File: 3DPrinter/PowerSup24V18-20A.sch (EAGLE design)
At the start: 77 parts, among them IC1 POWER-TNY264PN, T1 TRANS-1/1EFD25-10, T2 _TRANSFORMERS_GDT_20X6.5, T3 TRANS-1/1ETD39, U1 SG3525AN, X1 CON-7.62-02P, X2 CON-7.62-02P

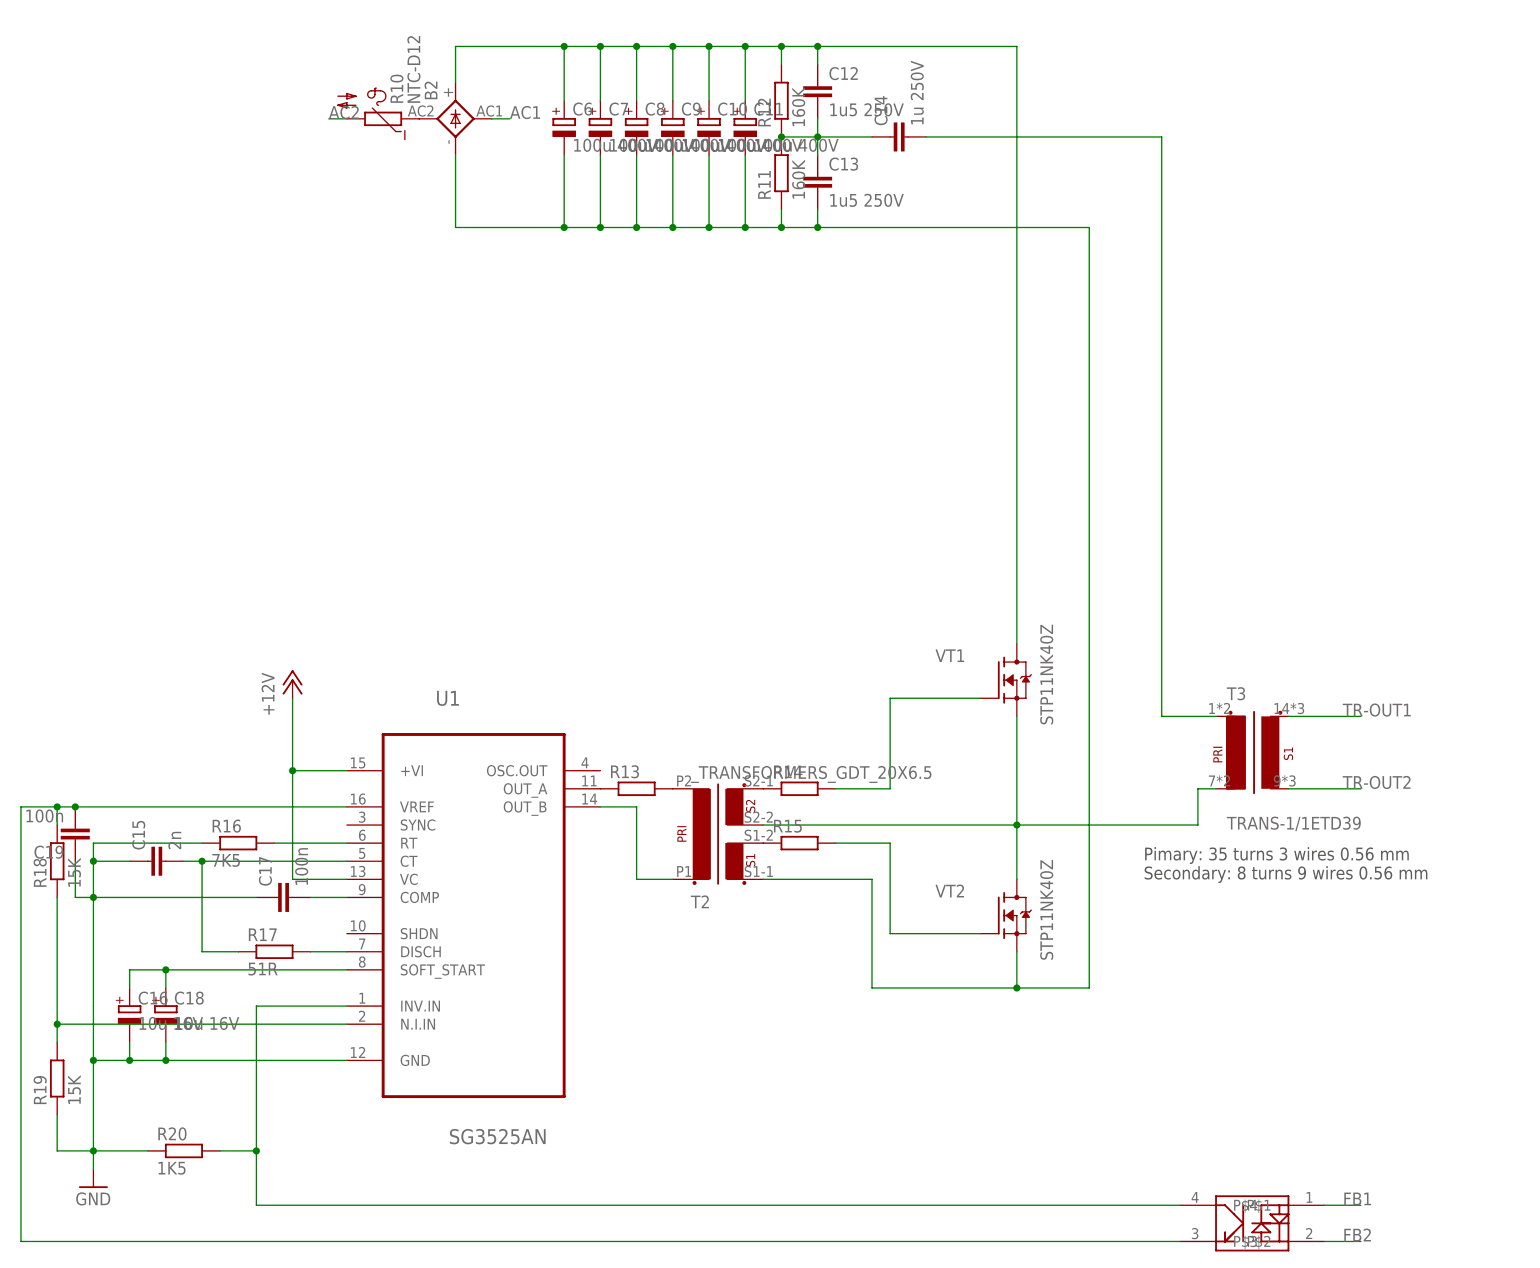
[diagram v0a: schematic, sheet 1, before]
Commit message: как всегда
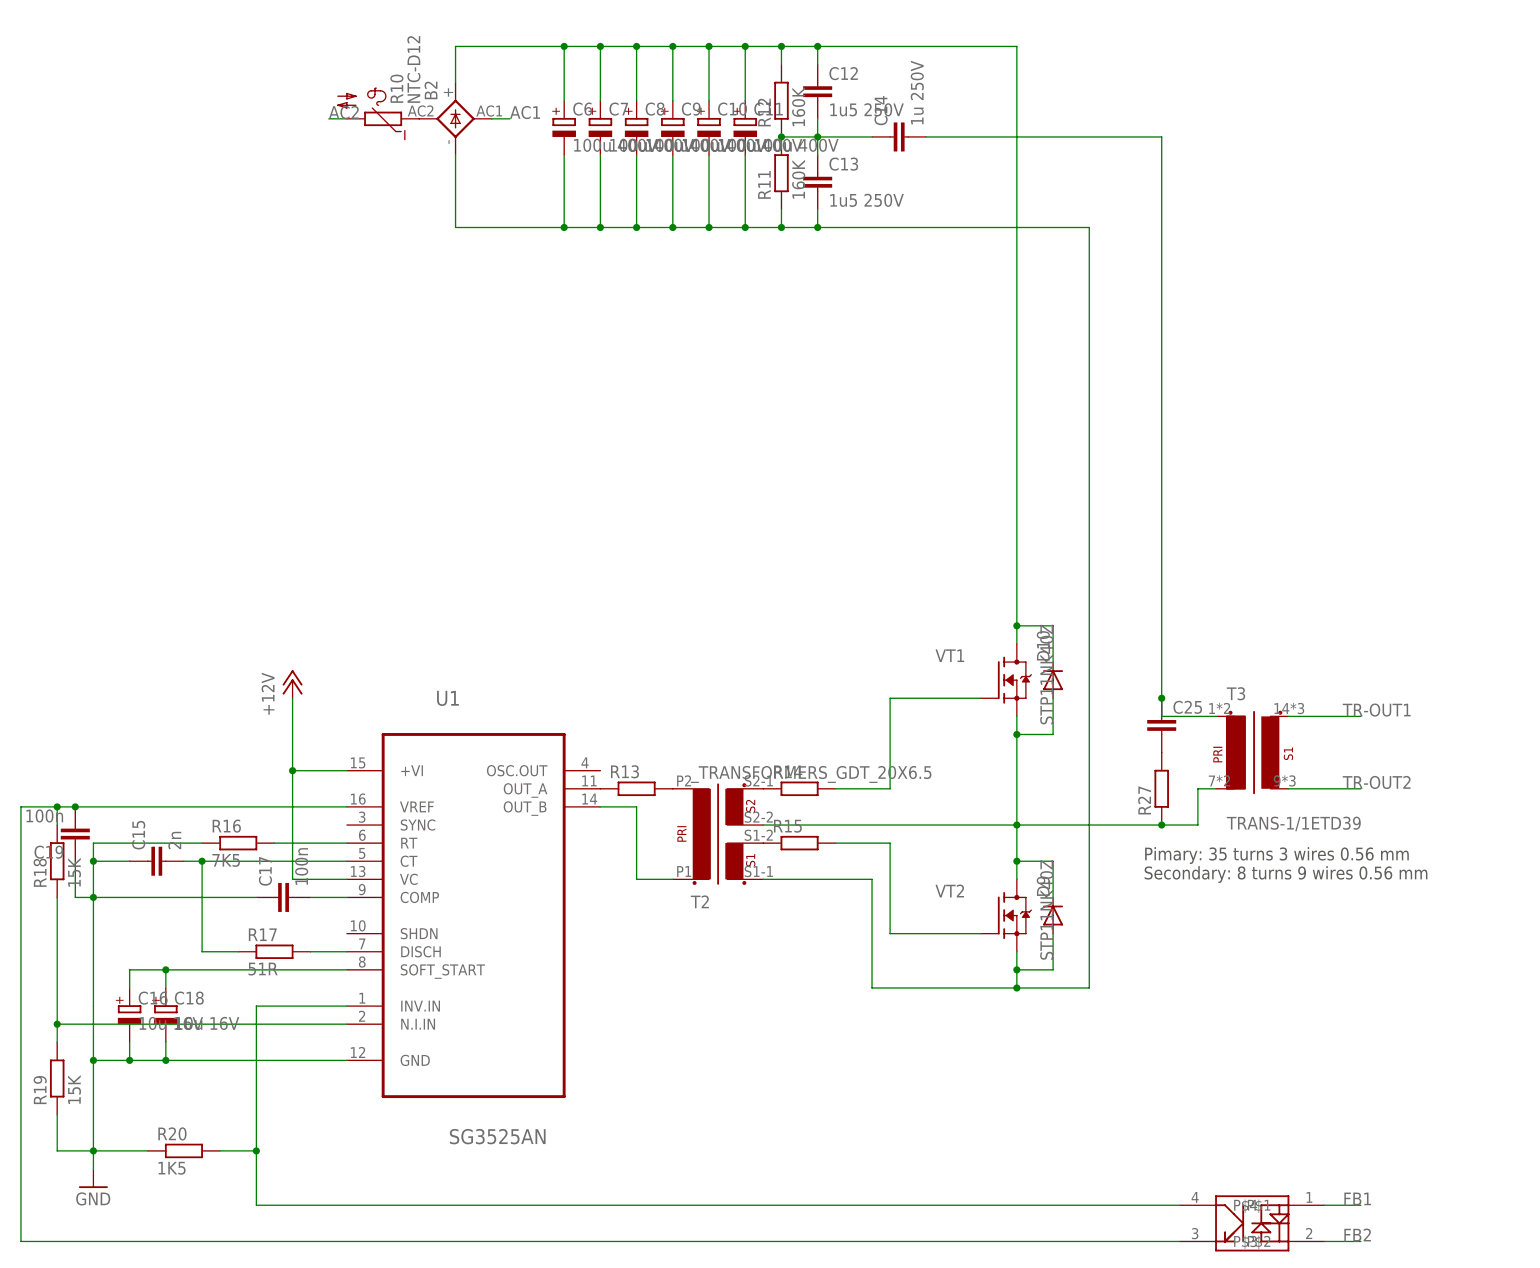
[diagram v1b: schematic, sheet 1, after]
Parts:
- added C25: (no value), Namenlos:CAP_C50-024X044
- added D10, D9: (no value), Namenlos:DIODE_ES1J
- added R27: (no value), Namenlos:R_MF-2
- C20, C21, C22, C23: device rcl:CPOL-EUE7.5-16 -> rcl:CPOL-EUE5-13
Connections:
- new net N$44: C25.2, R27.2
- net N$13: now also D10.C
- net N$19: now also D9.A
- net N$27: now also D10.A, D9.C, R27.1
- net N$28: now also C25.1
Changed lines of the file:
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@@
 <?xml version="1.0" encoding="utf-8"?>
 <!DOCTYPE eagle SYSTEM "eagle.dtd">
-<eagle version="8.3.2">
+<eagle version="8.3.1">
 <drawing>
 <settings>
@@
 <part name="JP2" library="pinhead" deviceset="PINHD-1X2" device=""/>
 <part name="L1" library="Namenlos" deviceset="INDUCTOR" device="D26.7"/>
-<part name="C20" library="rcl" library_urn="urn:adsk.eagle:library:334" deviceset="CPOL-EU" device="E7.5-16" package3d_urn="urn:adsk.eagle:package:23382/2"/>
-<part name="C21" library="rcl" library_urn="urn:adsk.eagle:library:334" deviceset="CPOL-EU" device="E7.5-16" package3d_urn="urn:adsk.eagle:package:23382/2"/>
-<part name="C22" library="rcl" library_urn="urn:adsk.eagle:library:334" deviceset="CPOL-EU" device="E7.5-16" package3d_urn="urn:adsk.eagle:package:23382/2"/>
-<part name="C23" library="rcl" library_urn="urn:adsk.eagle:library:334" deviceset="CPOL-EU" device="E7.5-16" package3d_urn="urn:adsk.eagle:package:23382/2"/>
+<part name="C20" library="rcl" library_urn="urn:adsk.eagle:library:334" deviceset="CPOL-EU" device="E5-13" package3d_urn="urn:adsk.eagle:package:23375/1"/>
+<part name="C21" library="rcl" library_urn="urn:adsk.eagle:library:334" deviceset="CPOL-EU" device="E5-13" package3d_urn="urn:adsk.eagle:package:23375/1"/>
+<part name="C22" library="rcl" library_urn="urn:adsk.eagle:library:334" deviceset="CPOL-EU" device="E5-13" package3d_urn="urn:adsk.eagle:package:23375/1"/>
+<part name="C23" library="rcl" library_urn="urn:adsk.eagle:library:334" deviceset="CPOL-EU" device="E5-13" package3d_urn="urn:adsk.eagle:package:23375/1"/>
 <part name="X2" library="Namenlos" deviceset="CON-7.62-02P" device=""/>
 <part name="TL2" library="Namenlos" deviceset="IC-TL431" device="CDBZR"/>
@@
 <part name="D8" library="Namenlos" deviceset="LED_" device="3MM"/>
 <part name="R26" library="Namenlos" deviceset="R_" device="0805" value="2K"/>
+<part name="R27" library="Namenlos" deviceset="R_" device="MF-2"/>
+<part name="C25" library="Namenlos" deviceset="CAP_" device="C50-024X044"/>
+<part name="D9" library="Namenlos" deviceset="DIODE_" device="ES1J"/>
+<part name="D10" library="Namenlos" deviceset="DIODE_" device="ES1J"/>
 </parts>
 <sheets>
@@
 <instance part="U$1" gate="G$1" x="144.78" y="-78.74" rot="MR0"/>
 <instance part="C19" gate="G$1" x="-20.32" y="-25.4" rot="R180"/>
+<instance part="R27" gate="G$1" x="132.08" y="-17.78" rot="R90"/>
+<instance part="C25" gate="G$1" x="132.08" y="-7.62"/>
+<instance part="D9" gate="G$1" x="116.84" y="-35.56" rot="R90"/>
+<instance part="D10" gate="G$1" x="116.84" y="-2.54" rot="R90"/>
 </instances>
 <busses>
@@
 <wire x1="33.02" y1="81.28" x2="33.02" y2="86.36" width="0.1524" layer="91"/>
 <pinref part="C10" gate="G$1" pin="+"/>
-<wire x1="33.02" y1="86.36" x2="43.18" y2="86.36" width="0.1524" layer="91"/>
-<wire x1="43.18" y1="86.36" x2="48.26" y2="86.36" width="0.1524" layer="91"/>
+<wire x1="33.02" y1="86.36" x2="48.26" y2="86.36" width="0.1524" layer="91"/>
 <wire x1="48.26" y1="86.36" x2="53.34" y2="86.36" width="0.1524" layer="91"/>
 <wire x1="53.34" y1="86.36" x2="58.42" y2="86.36" width="0.1524" layer="91"/>
@@
 <junction x="78.74" y="86.36"/>
 <pinref part="VT1" gate="G$1" pin="D"/>
-<wire x1="111.76" y1="2.54" x2="111.76" y2="86.36" width="0.1524" layer="91"/>
+<wire x1="111.76" y1="2.54" x2="111.76" y2="5.08" width="0.1524" layer="91"/>
+<wire x1="111.76" y1="5.08" x2="111.76" y2="86.36" width="0.1524" layer="91"/>
 <wire x1="111.76" y1="86.36" x2="83.82" y2="86.36" width="0.1524" layer="91"/>
 <junction x="83.82" y="86.36"/>
+<pinref part="D10" gate="G$1" pin="C"/>
+<wire x1="116.84" y1="0" x2="116.84" y2="5.08" width="0.1524" layer="91"/>
+<wire x1="116.84" y1="5.08" x2="111.76" y2="5.08" width="0.1524" layer="91"/>
+<junction x="111.76" y="5.08"/>
 </segment>
 </net>
@@
 <segment>
 <pinref part="B2" gate="1" pin="-"/>
-<wire x1="43.18" y1="60.96" x2="33.02" y2="60.96" width="0.1524" layer="91"/>
+<wire x1="48.26" y1="60.96" x2="33.02" y2="60.96" width="0.1524" layer="91"/>
 <wire x1="33.02" y1="60.96" x2="33.02" y2="71.12" width="0.1524" layer="91"/>
 <pinref part="C11" gate="G$1" pin="-"/>
-<wire x1="43.18" y1="60.96" x2="48.26" y2="60.96" width="0.1524" layer="91"/>
 <wire x1="48.26" y1="60.96" x2="53.34" y2="60.96" width="0.1524" layer="91"/>
 <wire x1="53.34" y1="60.96" x2="58.42" y2="60.96" width="0.1524" layer="91"/>
@@
 <junction x="78.74" y="60.96"/>
 <pinref part="VT2" gate="G$1" pin="S"/>
-<wire x1="111.76" y1="-40.64" x2="111.76" y2="-45.72" width="0.1524" layer="91"/>
+<wire x1="111.76" y1="-40.64" x2="111.76" y2="-43.18" width="0.1524" layer="91"/>
+<wire x1="111.76" y1="-43.18" x2="111.76" y2="-45.72" width="0.1524" layer="91"/>
 <wire x1="111.76" y1="-45.72" x2="121.92" y2="-45.72" width="0.1524" layer="91"/>
 <wire x1="121.92" y1="-45.72" x2="121.92" y2="60.96" width="0.1524" layer="91"/>
@@
 <pinref part="T2" gate="G$1" pin="S1-1"/>
 <wire x1="91.44" y1="-30.48" x2="76.2" y2="-30.48" width="0.1524" layer="91"/>
+<pinref part="D9" gate="G$1" pin="A"/>
+<wire x1="116.84" y1="-38.1" x2="116.84" y2="-43.18" width="0.1524" layer="91"/>
+<wire x1="116.84" y1="-43.18" x2="111.76" y2="-43.18" width="0.1524" layer="91"/>
+<junction x="111.76" y="-43.18"/>
 </segment>
 </net>
@@
 <wire x1="76.2" y1="-22.86" x2="111.76" y2="-22.86" width="0.1524" layer="91"/>
 <pinref part="VT2" gate="G$1" pin="D"/>
-<wire x1="111.76" y1="-22.86" x2="111.76" y2="-30.48" width="0.1524" layer="91"/>
+<wire x1="111.76" y1="-22.86" x2="111.76" y2="-27.94" width="0.1524" layer="91"/>
 <pinref part="VT1" gate="G$1" pin="S"/>
-<wire x1="111.76" y1="-22.86" x2="111.76" y2="-7.62" width="0.1524" layer="91"/>
+<wire x1="111.76" y1="-27.94" x2="111.76" y2="-30.48" width="0.1524" layer="91"/>
+<wire x1="111.76" y1="-22.86" x2="111.76" y2="-10.16" width="0.1524" layer="91"/>
 <junction x="111.76" y="-22.86"/>
+<wire x1="111.76" y1="-10.16" x2="111.76" y2="-7.62" width="0.1524" layer="91"/>
 <wire x1="137.16" y1="-17.78" x2="137.16" y2="-22.86" width="0.1524" layer="91"/>
-<wire x1="137.16" y1="-22.86" x2="111.76" y2="-22.86" width="0.1524" layer="91"/>
+<wire x1="137.16" y1="-22.86" x2="132.08" y2="-22.86" width="0.1524" layer="91"/>
 <pinref part="T3" gate="G$1" pin="P1-2"/>
+<wire x1="132.08" y1="-22.86" x2="111.76" y2="-22.86" width="0.1524" layer="91"/>
 <wire x1="137.16" y1="-17.78" x2="139.7" y2="-17.78" width="0.1524" layer="91"/>
+<pinref part="R27" gate="G$1" pin="1"/>
+<junction x="132.08" y="-22.86"/>
+<pinref part="D10" gate="G$1" pin="A"/>
+<wire x1="116.84" y1="-5.08" x2="116.84" y2="-10.16" width="0.1524" layer="91"/>
+<wire x1="116.84" y1="-10.16" x2="111.76" y2="-10.16" width="0.1524" layer="91"/>
+<junction x="111.76" y="-10.16"/>
+<pinref part="D9" gate="G$1" pin="C"/>
+<wire x1="116.84" y1="-33.02" x2="116.84" y2="-27.94" width="0.1524" layer="91"/>
+<wire x1="116.84" y1="-27.94" x2="111.76" y2="-27.94" width="0.1524" layer="91"/>
+<junction x="111.76" y="-27.94"/>
 </segment>
 </net>
@@
 <pinref part="C14" gate="G$1" pin="2"/>
 <wire x1="99.06" y1="73.66" x2="132.08" y2="73.66" width="0.1524" layer="91"/>
-<wire x1="132.08" y1="73.66" x2="132.08" y2="-7.62" width="0.1524" layer="91"/>
+<wire x1="132.08" y1="73.66" x2="132.08" y2="-5.08" width="0.1524" layer="91"/>
 <pinref part="T3" gate="G$1" pin="P1-1"/>
+<wire x1="132.08" y1="-5.08" x2="132.08" y2="-7.62" width="0.1524" layer="91"/>
 <wire x1="139.7" y1="-7.62" x2="132.08" y2="-7.62" width="0.1524" layer="91"/>
+<pinref part="C25" gate="G$1" pin="1"/>
+<junction x="132.08" y="-5.08"/>
 </segment>
 </net>
@@
 </segment>
 </net>
+<net name="N$44" class="0">
+<segment>
+<pinref part="R27" gate="G$1" pin="2"/>
+<pinref part="C25" gate="G$1" pin="2"/>
+</segment>
+</net>
